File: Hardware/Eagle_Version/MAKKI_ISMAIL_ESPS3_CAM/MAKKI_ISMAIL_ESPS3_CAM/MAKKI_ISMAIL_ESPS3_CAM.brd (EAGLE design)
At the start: 62.3 x 57.2 mm, 77 parts, among them IC1 LC709203F/MH, IC2 ESP32-S3-WROOM-1-N16R8, IC3 XC6206P282MR-G, IC4 ICS-43434, J1 2-2328702-4, J2 B2B-XH-A, Q1 DMG3415U, Q2 2N7002, Q3 DMG3415U, SW1 KMR2, SW2 KMR2, U1 MAX98357A, U2 AP2112/RT9080-3.3, U3 MCP73831T-2ACI/OT, X1 JSTPH, X3 USB C

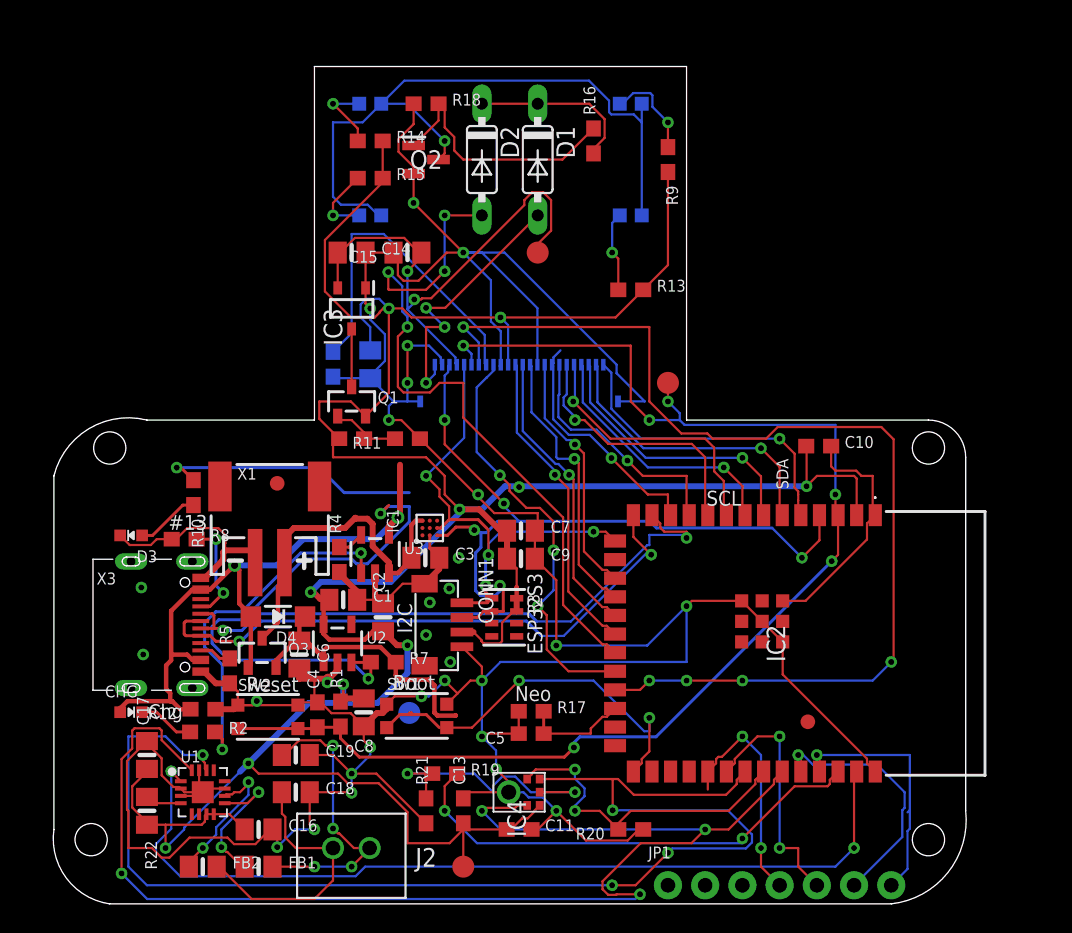
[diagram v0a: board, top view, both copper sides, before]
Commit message: Version Corrige
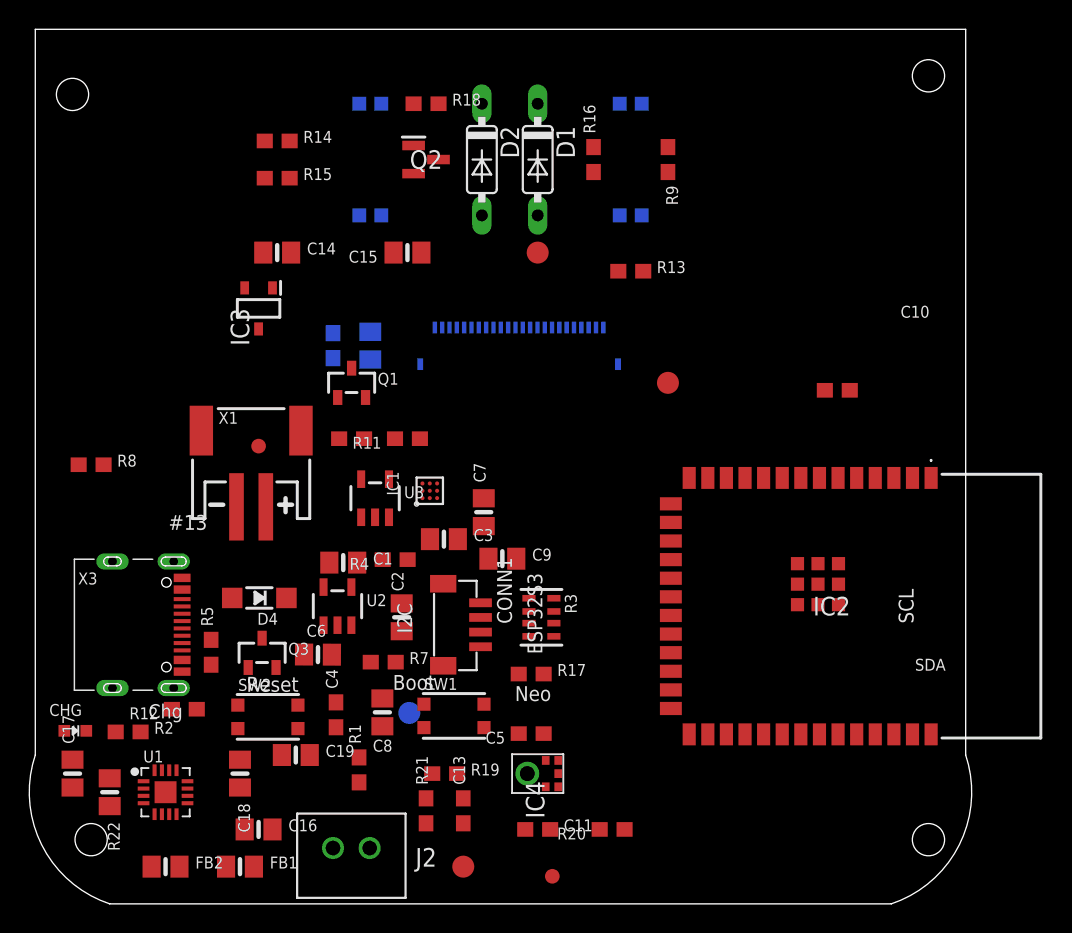
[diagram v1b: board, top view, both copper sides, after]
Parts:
- removed D3: RED, microbuilder:CHIPLED_0603_NOOUTLINE
- removed JP1: (no value), microbuilder:1X07_ROUND_76
- removed R10: 5.1K, microbuilder:0603-NO
- moved U$35 20.4 mm to (31.5, -1.93), turned to 180 degrees
- moved R8 8.13 mm to (0.00, 26.2)
- moved IC3 6.35 mm to (11.4, 36.8)
- moved R14 6.35 mm to (12.7, 48.3)
- moved R15 6.35 mm to (12.7, 45.7)
- moved C17 5.24 mm to (-1.27, 5.08)
- moved C14 5.08 mm to (12.7, 40.6)
- moved R2 5.08 mm to (2.53, 7.92)
- moved IC2 4.58 mm to (52.1, 16.5)
- moved C10 4.02 mm to (50.9, 31.2)
- moved X1 4.02 mm to (10.9, 27.0)
- moved C18 4.02 mm to (10.2, 5.08), turned to 270 degrees
- moved CHG 4.02 mm to (-1.08, 8.00)
- moved R1 4.02 mm to (18.3, 5.33)
- moved U3 3.81 mm to (19.4, 23.9)
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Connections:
- removed net 1.8V: IC2.25
- removed net D13: R10.1
- removed net D8: IC2.18, J1.14
- removed net D9: IC2.20, J1.12
- removed net N$5: D3.A, R10.2
- removed net RX: IC2.31, JP1.4
- removed net TX: IC2.32, JP1.5
- net D7: now also IC2.31; no longer IC2.17
- net GND: no longer D3.C
- net RESET: no longer J1.6
- net RXD0: no longer JP1.6
- net TXD0: no longer JP1.7
- net XVCLK: now also IC2.32; no longer IC2.19
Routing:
- net GND: track 320.6 -> 0.00 mm, vias 30 -> 0
- net 3.3V: track 223.8 -> 0.00 mm, vias 9 -> 0
- net RESET: track 91.5 -> 0.00 mm, vias 6 -> 0
- net BCLK: track 89.8 -> 0.00 mm, vias 4 -> 0
- net WS: track 88.1 -> 0.00 mm, vias 4 -> 0
- net VSYNC: track 74.1 -> 0.00 mm, vias 5 -> 0
- net DIN: track 61.3 -> 0.00 mm, vias 2 -> 0
- net SDA: track 54.2 -> 0.00 mm, vias 5 -> 0
- net COMMAND: track 48.3 -> 0.00 mm, vias 4 -> 0
- net N$13: track 47.2 -> 0.00 mm, vias 1 -> 0
- net VBUS: track 44.8 -> 0.00 mm, vias 2 -> 0
- net D-: track 42.5 -> 0.00 mm, vias 2 -> 0
- net D+: track 40.9 -> 0.00 mm, vias 2 -> 0
- net EN: track 36.0 -> 0.00 mm, vias 2 -> 0
- net 2.8V: track 36.0 -> 0.00 mm, vias 2 -> 0
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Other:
- board size 62.3 x 57.2 mm -> 64.3 x 59.7 mm
